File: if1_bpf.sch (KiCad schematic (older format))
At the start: 8 parts

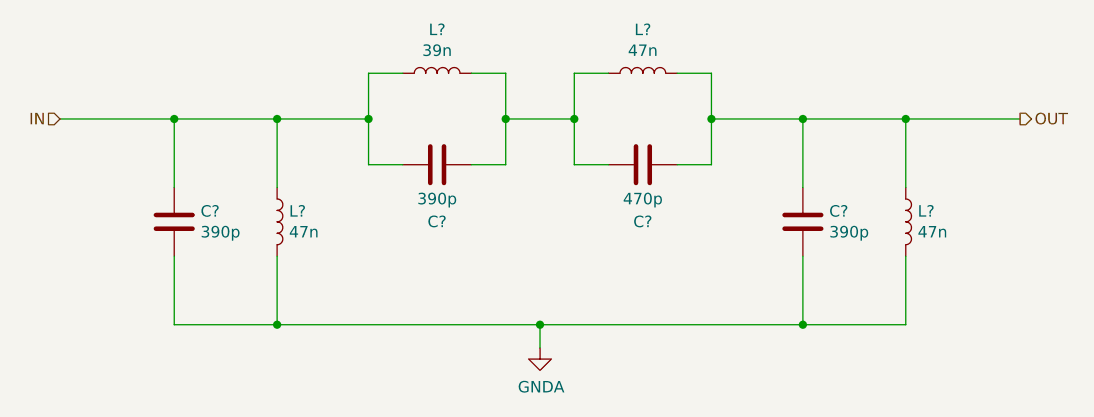
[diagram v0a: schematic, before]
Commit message: Footprint reassociation, pcb clear
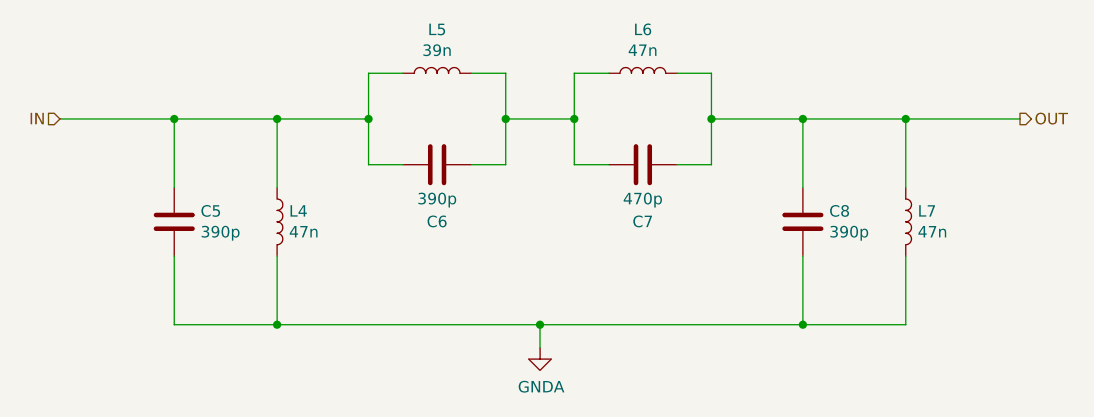
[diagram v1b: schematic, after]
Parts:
- C5, C6, C7, C8: renamed from C?; footprint (none) -> Capacitor_SMD:C_0805_2012Metric_Pad1.18x1.45mm_HandSolder
- L4, L6, L7: renamed from L?; footprint (none) -> Inductor_SMD:L_0603_1608Metric_Pad1.05x0.95mm_HandSolder
- L5: renamed from L?; footprint (none) -> Inductor_SMD:L_0402_1005Metric_Pad0.77x0.64mm_HandSolder
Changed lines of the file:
@@
 OUT
 $Comp
-L Device:C C?
+L Device:C C5
 U 1 1 600431FC
 P 4450 3850
-F 0 "C?" H 4565 3896 50  0000 L CNN
+F 0 "C5" H 4565 3896 50  0000 L CNN
 F 1 "390p" H 4565 3805 50  0000 L CNN
-F 2 "" H 4488 3700 50  0001 C CNN
+F 2 "Capacitor_SMD:C_0805_2012Metric_Pad1.18x1.45mm_HandSolder" H 4488 3700 50  0001 C CNN
 F 3 "~" H 4450 3850 50  0001 C CNN
 	1    4450 3850
@@
 $EndComp
 $Comp
-L Device:L L?
+L Device:L L4
 U 1 1 600436A2
 P 4900 3850
-F 0 "L?" H 4952 3896 50  0000 L CNN
+F 0 "L4" H 4952 3896 50  0000 L CNN
 F 1 "47n" H 4952 3805 50  0000 L CNN
-F 2 "" H 4900 3850 50  0001 C CNN
+F 2 "Inductor_SMD:L_0603_1608Metric_Pad1.05x0.95mm_HandSolder" H 4900 3850 50  0001 C CNN
 F 3 "~" H 4900 3850 50  0001 C CNN
 F 4 "93-02-59" H 4900 3850 50  0001 C CNN "Lomex"
@@
 $EndComp
 $Comp
-L Device:L L?
+L Device:L L5
 U 1 1 600471E0
 P 5600 3200
-F 0 "L?" V 5790 3200 50  0000 C CNN
+F 0 "L5" V 5790 3200 50  0000 C CNN
 F 1 "39n" V 5699 3200 50  0000 C CNN
-F 2 "" H 5600 3200 50  0001 C CNN
+F 2 "Inductor_SMD:L_0402_1005Metric_Pad0.77x0.64mm_HandSolder" H 5600 3200 50  0001 C CNN
 F 3 "~" H 5600 3200 50  0001 C CNN
 F 4 "2846682RL" H 5600 3200 50  0001 C CNN "Farnell"
@@
 $EndComp
 $Comp
-L Device:C C?
+L Device:C C6
 U 1 1 6004779D
 P 5600 3600
-F 0 "C?" V 5350 3600 50  0000 C CNN
+F 0 "C6" V 5350 3600 50  0000 C CNN
 F 1 "390p" V 5450 3600 50  0000 C CNN
-F 2 "" H 5638 3450 50  0001 C CNN
+F 2 "Capacitor_SMD:C_0805_2012Metric_Pad1.18x1.45mm_HandSolder" H 5638 3450 50  0001 C CNN
 F 3 "~" H 5600 3600 50  0001 C CNN
 	1    5600 3600
@@
 $EndComp
 $Comp
-L Device:L L?
+L Device:L L6
 U 1 1 6004D573
 P 6500 3200
-F 0 "L?" V 6690 3200 50  0000 C CNN
+F 0 "L6" V 6690 3200 50  0000 C CNN
 F 1 "47n" V 6599 3200 50  0000 C CNN
-F 2 "" H 6500 3200 50  0001 C CNN
+F 2 "Inductor_SMD:L_0603_1608Metric_Pad1.05x0.95mm_HandSolder" H 6500 3200 50  0001 C CNN
 F 3 "~" H 6500 3200 50  0001 C CNN
 F 4 "93-02-59" H 6500 3200 50  0001 C CNN "Lomex"
@@
 $EndComp
 $Comp
-L Device:C C?
+L Device:C C7
 U 1 1 6004D579
 P 6500 3600
-F 0 "C?" V 6250 3600 50  0000 C CNN
+F 0 "C7" V 6250 3600 50  0000 C CNN
 F 1 "470p" V 6350 3600 50  0000 C CNN
-F 2 "" H 6538 3450 50  0001 C CNN
+F 2 "Capacitor_SMD:C_0805_2012Metric_Pad1.18x1.45mm_HandSolder" H 6538 3450 50  0001 C CNN
 F 3 "~" H 6500 3600 50  0001 C CNN
 	1    6500 3600
@@
 $EndComp
 $Comp
-L Device:C C?
+L Device:C C8
 U 1 1 6004E74D
 P 7200 3850
-F 0 "C?" H 7315 3896 50  0000 L CNN
+F 0 "C8" H 7315 3896 50  0000 L CNN
 F 1 "390p" H 7315 3805 50  0000 L CNN
-F 2 "" H 7238 3700 50  0001 C CNN
+F 2 "Capacitor_SMD:C_0805_2012Metric_Pad1.18x1.45mm_HandSolder" H 7238 3700 50  0001 C CNN
 F 3 "~" H 7200 3850 50  0001 C CNN
 	1    7200 3850
@@
 $EndComp
 $Comp
-L Device:L L?
+L Device:L L7
 U 1 1 6004E753
 P 7650 3850
-F 0 "L?" H 7702 3896 50  0000 L CNN
+F 0 "L7" H 7702 3896 50  0000 L CNN
 F 1 "47n" H 7702 3805 50  0000 L CNN
-F 2 "" H 7650 3850 50  0001 C CNN
+F 2 "Inductor_SMD:L_0603_1608Metric_Pad1.05x0.95mm_HandSolder" H 7650 3850 50  0001 C CNN
 F 3 "~" H 7650 3850 50  0001 C CNN
 F 4 "93-02-59" H 7650 3850 50  0001 C CNN "Lomex"
@@
 	6050 4300 7200 4300
 $Comp
-L power:GNDA #PWR?
+L power:GNDA #PWR0108
 U 1 1 60071173
 P 6050 4400
-F 0 "#PWR?" H 6050 4150 50  0001 C CNN
+F 0 "#PWR0108" H 6050 4150 50  0001 C CNN
 F 1 "GNDA" H 6055 4227 50  0000 C CNN
 F 2 "" H 6050 4400 50  0001 C CNN
